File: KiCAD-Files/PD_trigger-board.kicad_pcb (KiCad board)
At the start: 2 copper layers, 18 x 23.5 mm, 16 parts, among them J1 USB_C_Receptacle_USB3.0_12P, U1 HUSB238, U2 SI4459ADY-T1-GE3, U3 ESP32-S3-mini_pinprofile

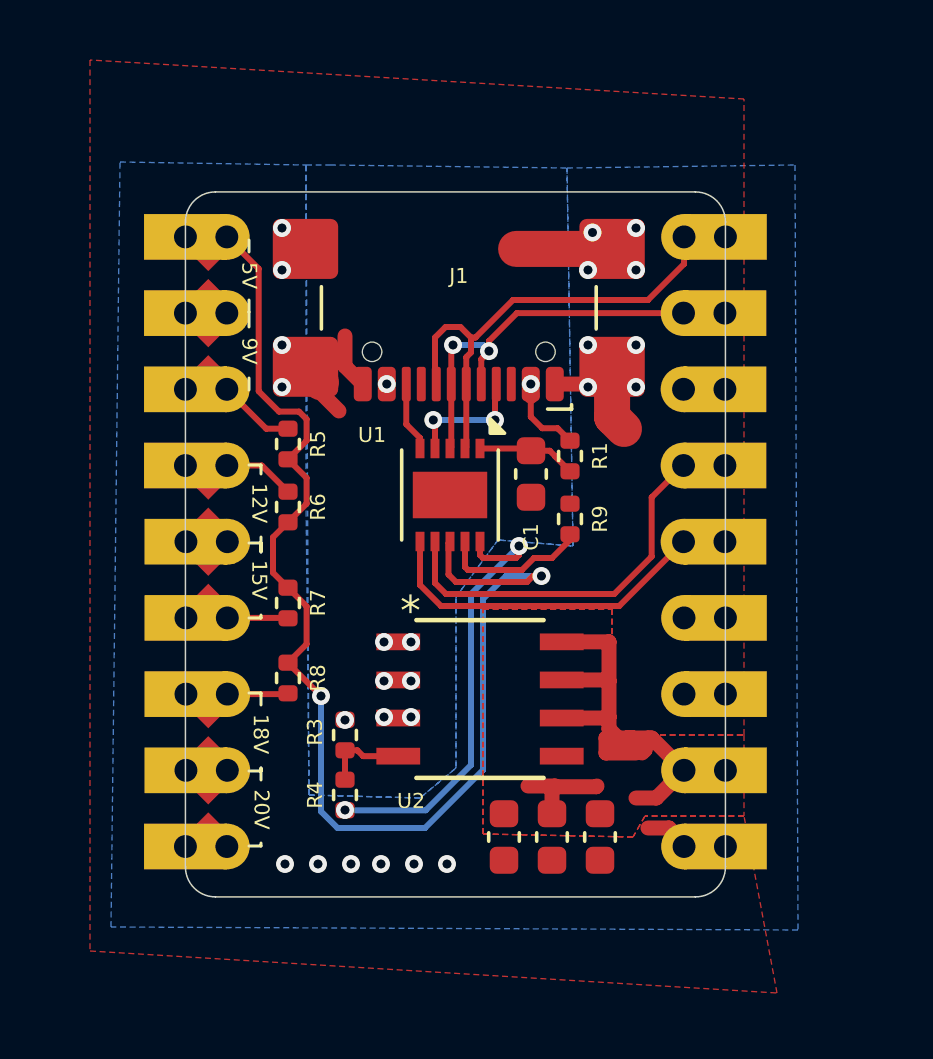
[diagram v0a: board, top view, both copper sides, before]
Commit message: Minor design changes
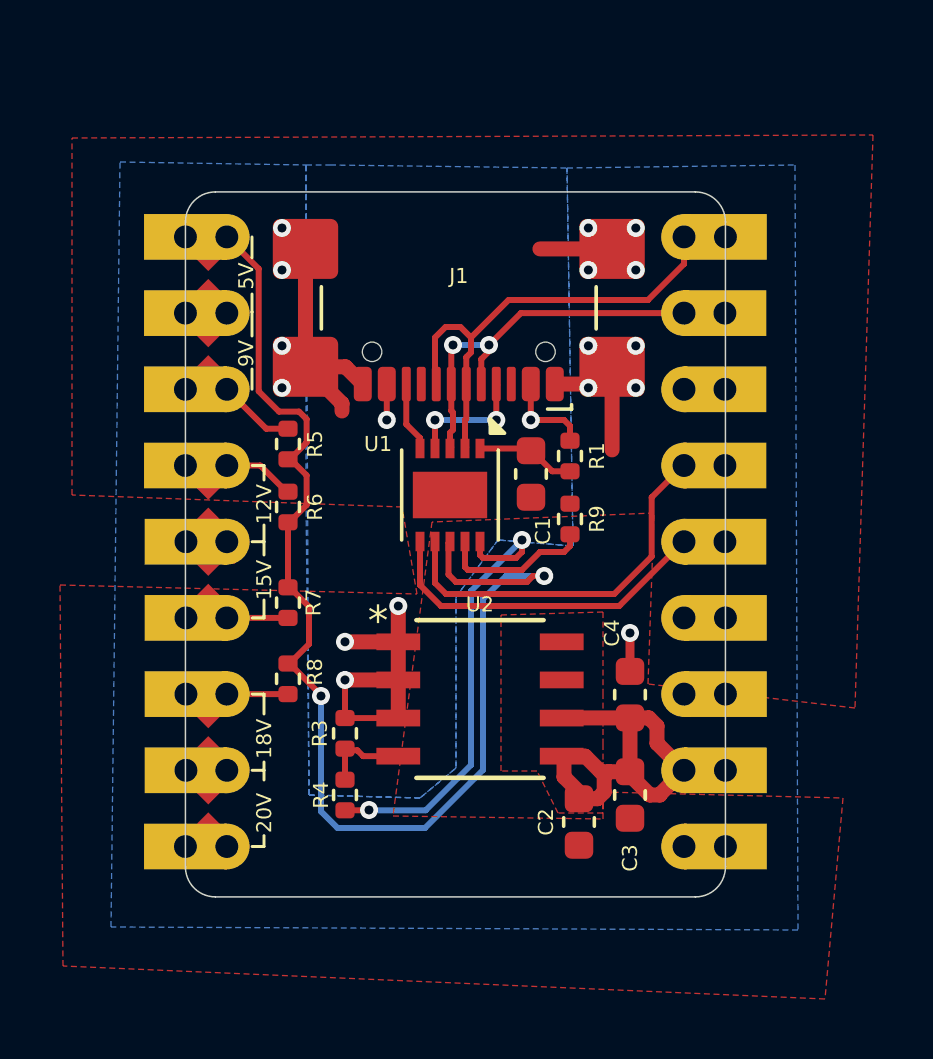
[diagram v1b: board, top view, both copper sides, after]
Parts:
- moved C4 4.85 mm to (145.9, 92.9), turned to 90 degrees
- moved C3 2.95 mm to (145.9, 96.2)
- moved C2 2.55 mm to (144.2, 97.1)
- moved R3 0.06 mm to (136.4, 94.1)
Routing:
- net VBUS: track 6.80 -> 15.9 mm, vias 9 -> 5
- net GND: track 30.9 -> 22.7 mm, vias 18 -> 13
- net VOUT: track 19.0 -> 15.5 mm

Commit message: minor changes for v0.2
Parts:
- added ce-symbol_mask_3mm: G***, blinkyparts:ce-icon_3mm, B.Cu at (145.2, 90.2)
- added rohs-symbol_mask_3mm: G***, blinkyparts:rohs-icon_3mm, B.Cu at (139.0, 86.4)
- added weee-symbol_mask_3mm: G***, blinkyparts:weee-icon_3mm, B.Cu at (139.5, 90.8)
